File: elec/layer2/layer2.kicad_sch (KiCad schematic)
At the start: 47 parts, among them J1 Conn_01x03, J10 Conn_01x05, J11 Conn_01x05, J12 XT60-M, J17 Conn_01x02, J18 Conn_01x02, J19 XT30UPB-M, J2 XT30UPB-M, J3 Conn_01x04, J4 Conn_01x05, J5 Conn_01x03, J6 XT30UPB-M, J7 XT30UPB-M, J9 XT30PW-M, SW1 SW_SPDT_312, U1 TEENSY40

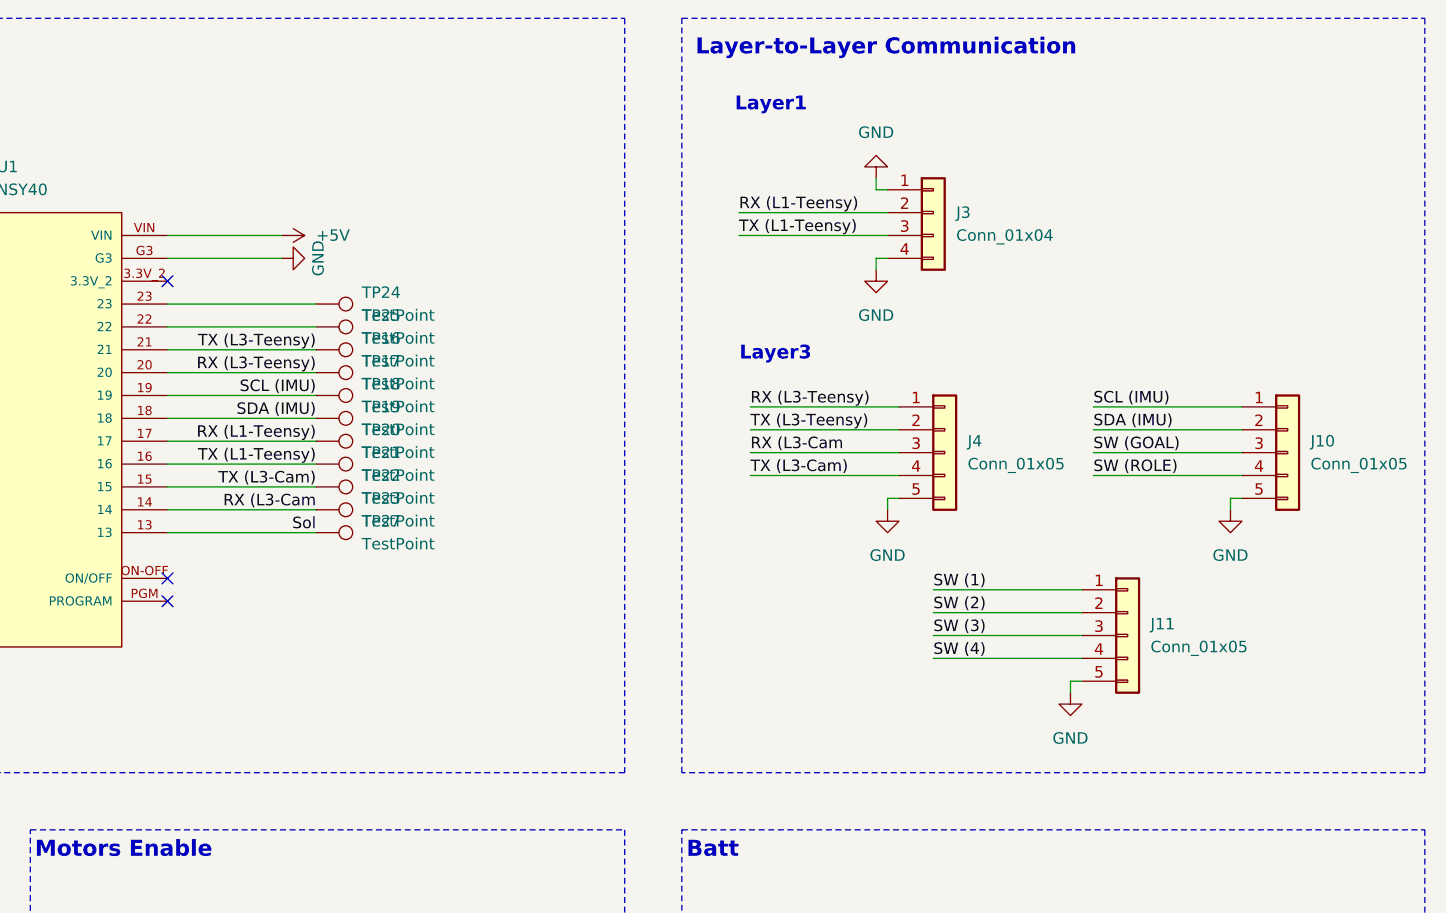
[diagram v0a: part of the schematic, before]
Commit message: fix: l2
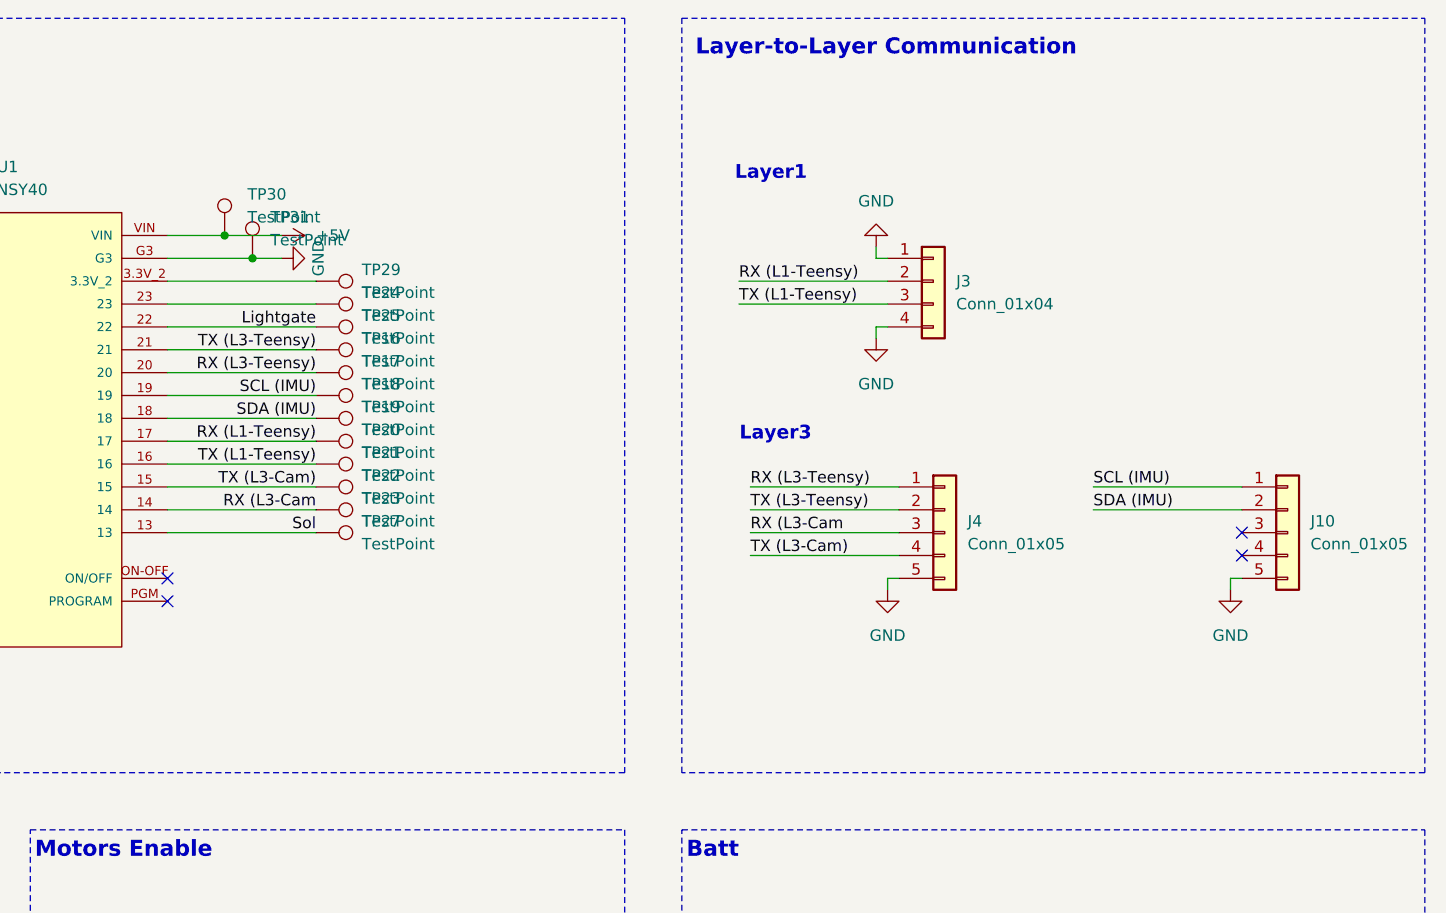
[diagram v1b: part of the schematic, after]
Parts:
- removed J11: Conn_01x05, Connector_JST:JST_XH_B5B-XH-A_1x05_P2.50mm_Vertical, symbol Connector_Generic:Conn_01x05
- added TP29, TP30, TP31: TestPoint, TestPoint:TestPoint_THTPad_D1.5mm_Drill0.7mm, symbol Connector:TestPoint
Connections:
- net +5V: now also TP30.1
- net GND: now also TP31.1
- net Lightgate: now also TP25.1, U1.22
- net at U1.3.3V_2: now also TP29.1
- net SW (GOAL): no longer names the net of J10.3 (Pin_3)
- net SW (ROLE): no longer names the net of J10.4 (Pin_4)
- no-connect marks 5 -> 6
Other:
- moved on the sheet: J10, J3, J4
